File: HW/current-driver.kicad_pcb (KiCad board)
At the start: 2 copper layers, 55 x 55 mm, 24 parts, among them P1 IN+, P2 IN-, P3 LED, P4 SW_IN, P5 SENSE, P6 OUT+, P7 OUT-, Q1 IRFZ44VBF, U1 INA168

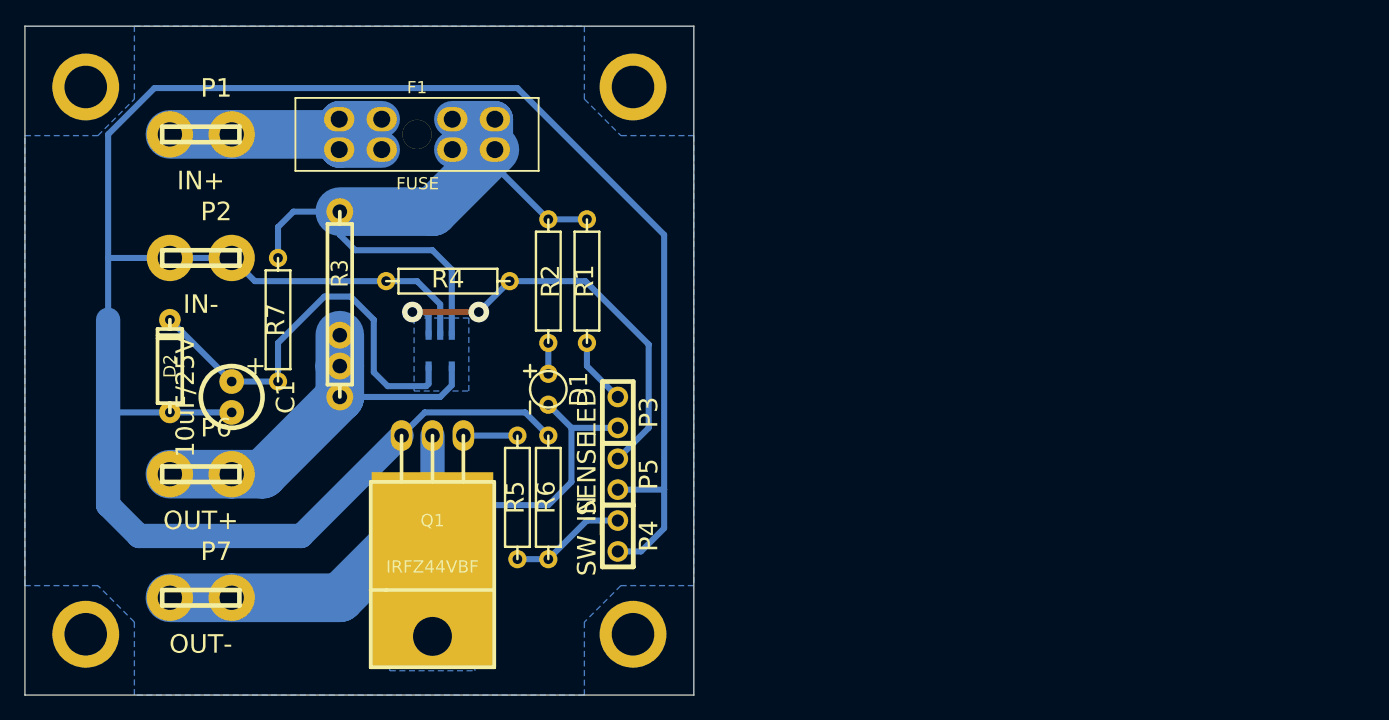
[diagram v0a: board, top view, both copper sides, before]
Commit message: final 5x5 pcb
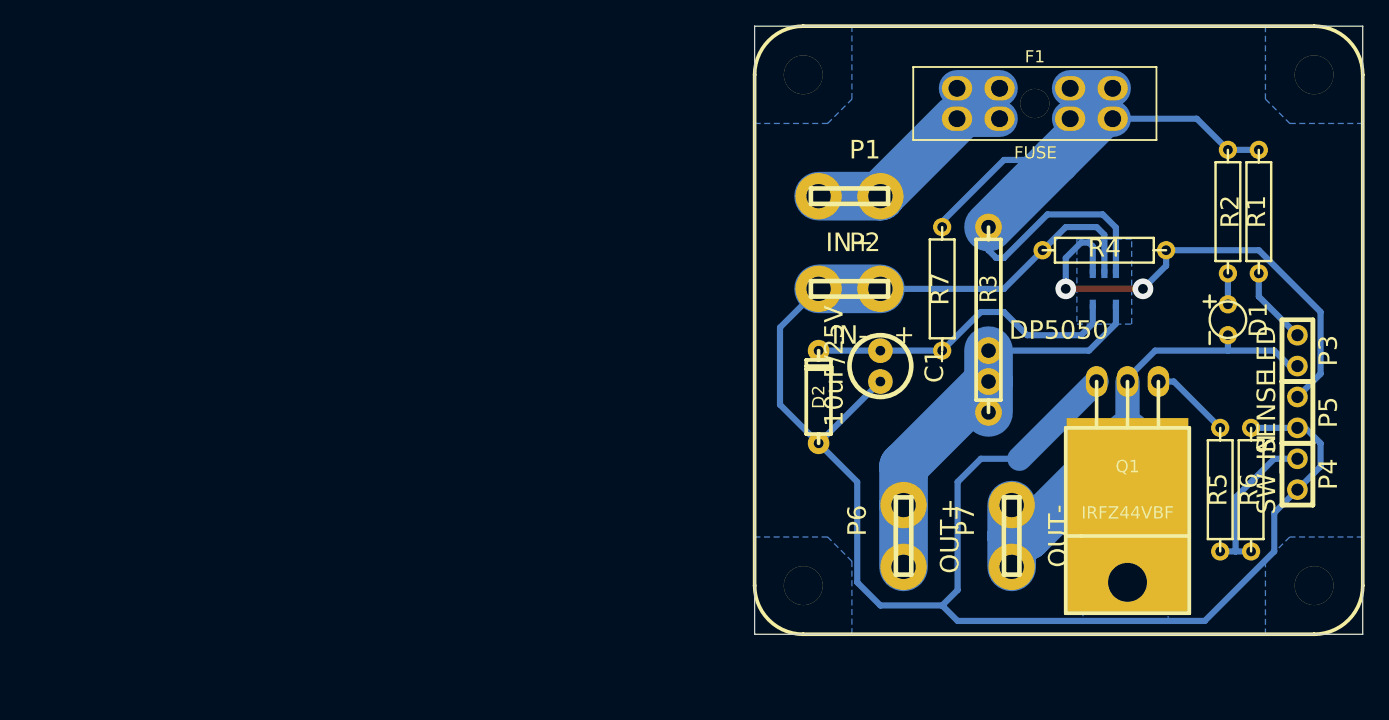
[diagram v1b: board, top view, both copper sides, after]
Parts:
- removed MNT_HOLE_3.5 (x4): , MNT_HOLE_3.5
- added DP5050: , DP5050, F.Cu at (195.0, 105.0)
- moved P7 66.9 mm to (191.1, 121.9), turned to 90 degrees
- moved P6 58.0 mm to (182.2, 121.9), turned to 90 degrees
- moved R5 57.8 mm to (208.3, 118.1)
- moved R6 57.8 mm to (210.8, 118.1)
- moved Q1 57.3 mm to (200.7, 109.2)
- moved D1 56.2 mm to (208.9, 104.1)
- moved R2 56.2 mm to (208.9, 95.2)
- moved P3 56.1 mm to (214.6, 106.7)
- moved P4 56.1 mm to (214.6, 116.8)
- moved P5 56.1 mm to (214.6, 111.8)
- moved R1 55.5 mm to (211.5, 95.2)
- moved U1 54.8 mm to (198.8, 101.6)
- moved R7 54.7 mm to (185.4, 101.6)
- moved R4 54.0 mm to (198.8, 98.4)
- moved P1 53.6 mm to (177.8, 94.0)
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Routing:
- net N-000006: track 199.1 -> 144.5 mm
- net N-000007: track 53.6 -> 39.4 mm
- net N-000004: track 35.2 -> 26.6 mm
- net N-0000011: track 60.9 -> 65.9 mm
- net N-000003: track 36.1 -> 40.5 mm
- net N-000002: track 9.57 -> 13.4 mm
- net N-000008: track 32.9 -> 36.2 mm
- net N-000001: track 4.44 -> 6.66 mm
- net N-000005: track 5.50 -> 6.40 mm
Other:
- board size 55 x 55 mm -> 50 x 50 mm
